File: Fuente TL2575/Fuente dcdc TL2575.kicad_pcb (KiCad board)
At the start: 2 copper layers, 53.3 x 35.6 mm, 20 parts, among them U1 TL2575

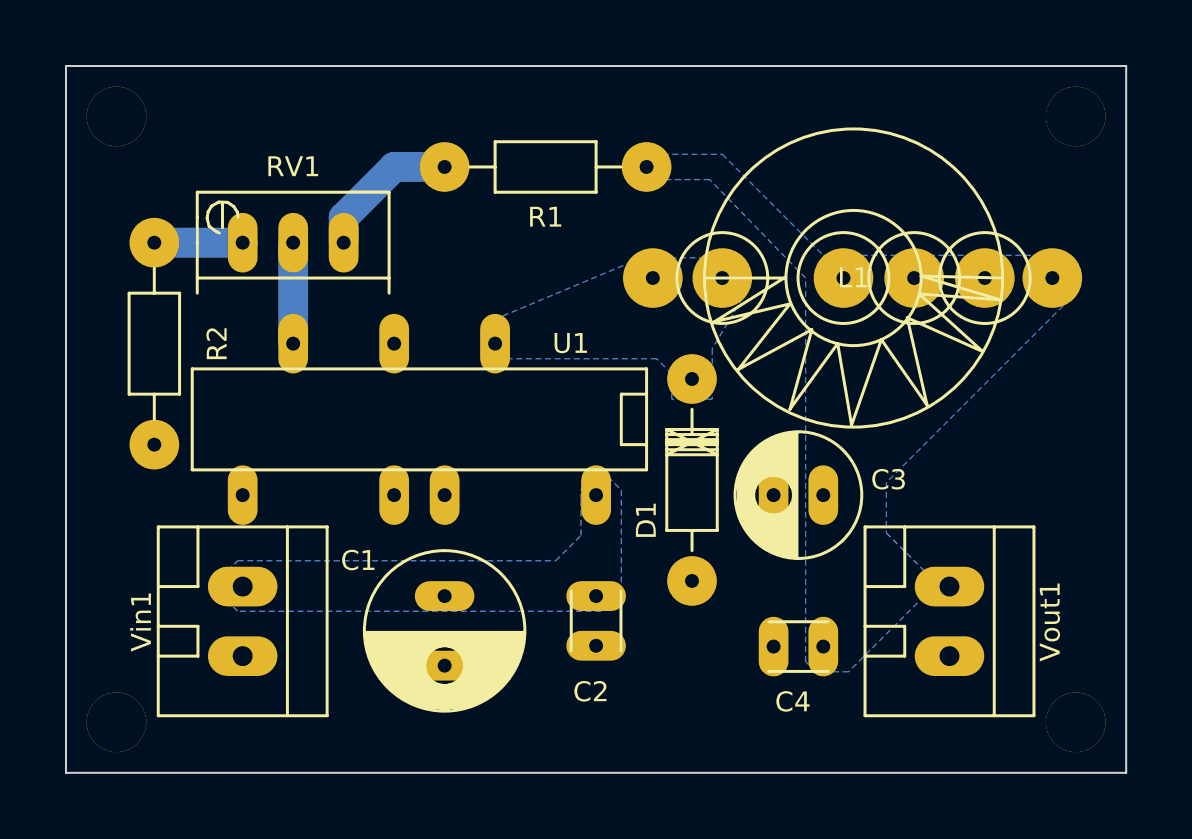
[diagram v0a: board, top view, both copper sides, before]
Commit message: Terminada Fuente TL2575, y controlador
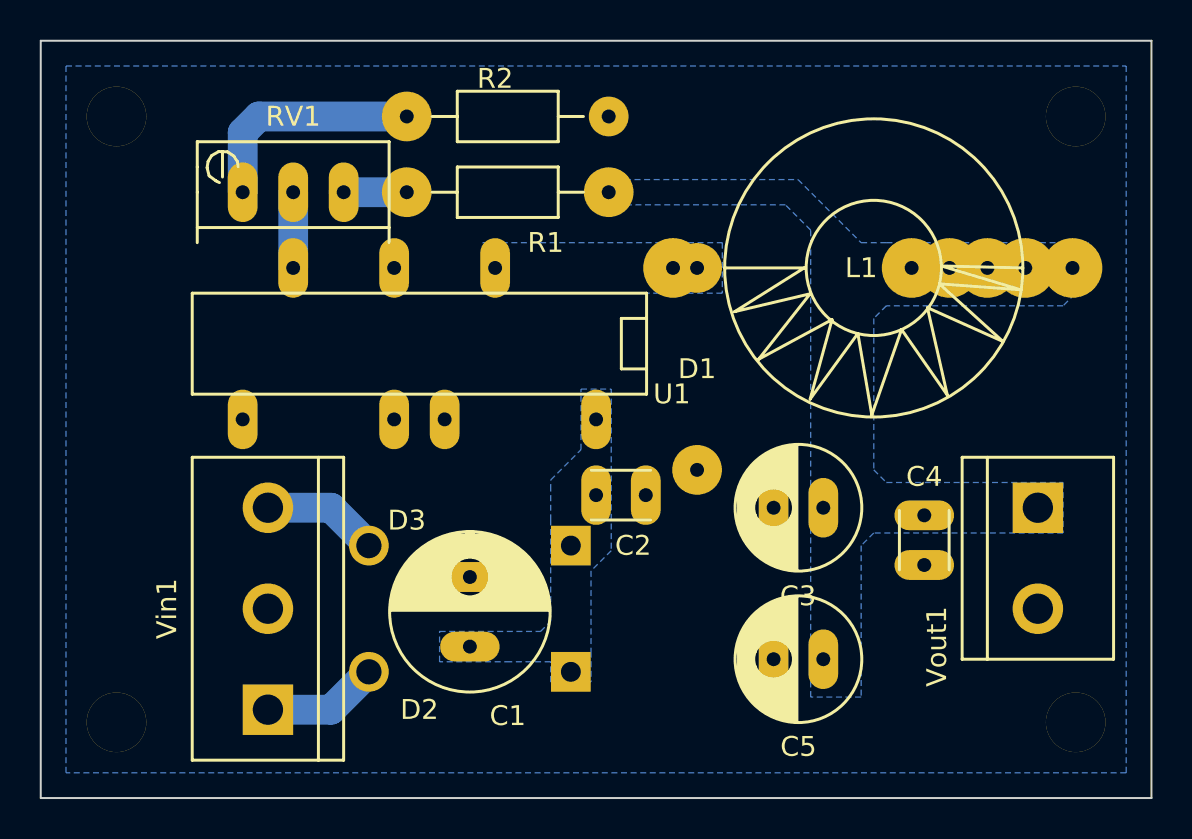
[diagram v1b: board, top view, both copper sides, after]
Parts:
- removed the REF** at (138.2, 48.8)
- removed the REF** at (141.7, 48.8)
- removed the REF** at (145.3, 48.8)
- removed the REF** at (132.1, 48.8)
- added C5: 100uF, Capacitors_ThroughHole:C_Radial_D6.3_L11.2_P2.5, F.Cu at (137.2, 67.9)
- added D2: D, Diodes_ThroughHole:Diode_DO-41_SOD81_Horizontal_RM10, B.Cu at (119.4, 68.6)
- added D3: D, Diodes_ThroughHole:Diode_DO-41_SOD81_Horizontal_RM10, B.Cu at (119.4, 62.2)
- added REF**: 1pin, Connect:1pin, F.Cu at (145.4, 48.3)
- added REF**: 1pin, Connect:1pin, F.Cu at (147.3, 48.3)
- added REF**: 1pin, Connect:1pin, F.Cu at (143.5, 48.3)
- added REF**: 1pin, Connect:1pin, F.Cu at (141.6, 48.3)
- D1: moved to B.Cu
- Vin1: value CONN_01X02 -> CONN_01X03; footprint Sockets_WAGO734:WAGO_734_2pin_Straight_RuggedPads -> Connect:bornier3
- Vout1: footprint Sockets_WAGO734:WAGO_734_2pin_Straight_RuggedPads -> Connect:bornier2
- moved R2 21.1 mm to (121.3, 40.6), turned to 0 degrees
- moved C4 8.33 mm to (142.2, 60.7), turned to 270 degrees
- moved D1 5.59 mm to (130.8, 53.3)
- moved Vout1 5.46 mm to (148.0, 62.9)
- moved C2 5.08 mm to (125.7, 59.7), turned to 0 degrees
- moved U1 3.81 mm to (116.8, 52.1)
- moved C1 2.84 mm to (119.4, 67.3), turned to 90 degrees
- moved RV1 2.54 mm to (108.0, 44.5)
- moved R1 2.29 mm to (121.3, 44.5)
- moved Vin1 1.42 mm to (109.2, 65.4), turned to 90 degrees
- moved L1 1.14 mm to (139.7, 48.3)
- moved C3 0.64 mm to (137.2, 60.3)
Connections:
- Vin1 pad 1: Net-(C1-Pad1) -> Net-(D2-Pad1)
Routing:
- net Net-(R2-Pad1): track 4.45 -> 11.6 mm
- net Net-(D2-Pad1): track 0.00 -> 5.87 mm
- net Net-(D3-Pad1): track 0.00 -> 5.87 mm
- net Net-(R1-Pad2): track 7.40 -> 3.17 mm
- net Net-(RV1-Pad2): track 5.08 -> 3.81 mm
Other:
- board size 53.3 x 35.6 mm -> 55.9 x 38.1 mm

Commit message: Para imprimir, fuente TL2575 y Controlador
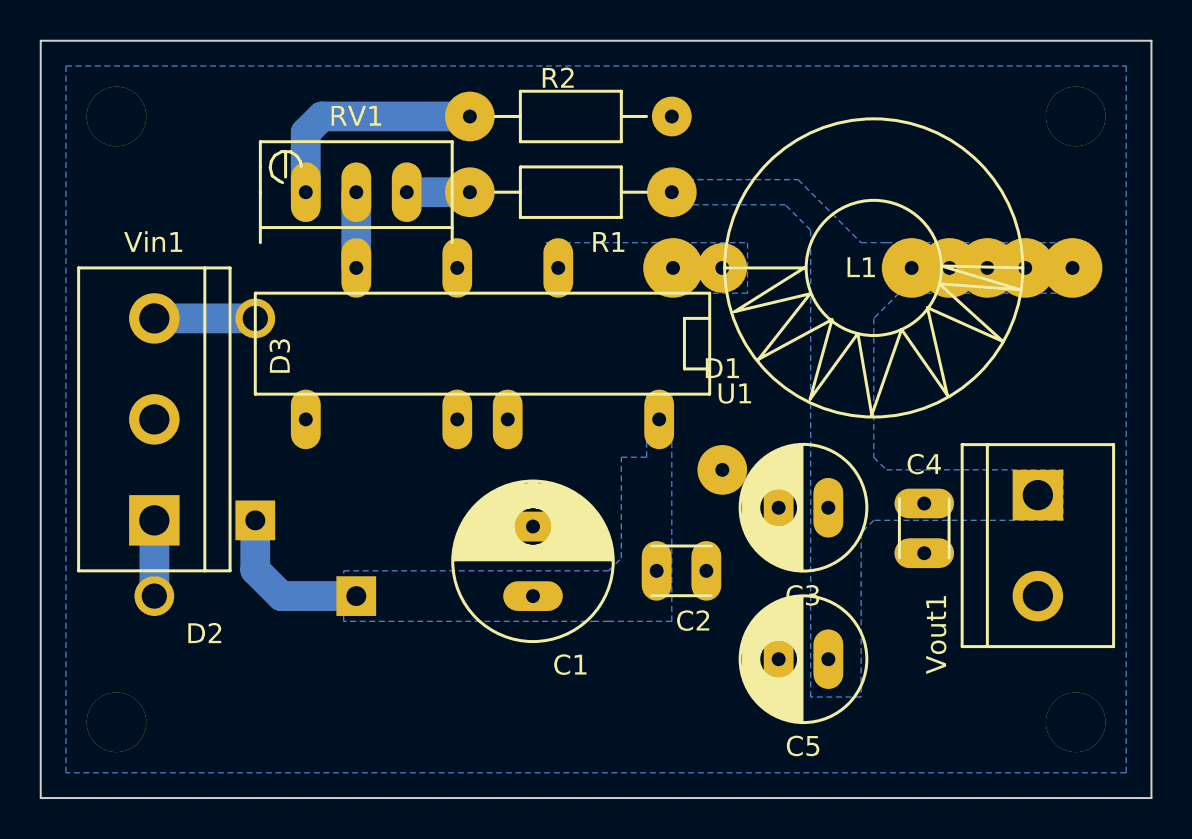
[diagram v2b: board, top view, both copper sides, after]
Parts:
- moved D3 12.5 mm to (108.6, 55.9), turned to 270 degrees
- moved D2 11.4 mm to (108.6, 64.8)
- moved Vin1 11.1 mm to (103.5, 55.9)
- moved C2 4.88 mm to (128.8, 63.5)
- moved C1 4.07 mm to (122.6, 64.8)
- moved R1 3.17 mm to (124.5, 44.5)
- moved R2 3.17 mm to (124.5, 40.6)
- moved RV1 3.17 mm to (111.1, 44.5)
- moved U1 3.17 mm to (120.0, 52.1)
- moved D1 1.27 mm to (132.1, 53.3)
- moved Vout1 0.64 mm to (148.0, 62.2)
- moved C4 0.60 mm to (142.2, 60.1)
- moved C3 0.25 mm to (137.4, 60.3)
- moved C5 0.25 mm to (137.4, 67.9)
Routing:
- net (no net): track 0.00 -> 53.3 mm
- net Net-(C1-Pad1): track 0.00 -> 8.12 mm
- net Net-(D2-Pad1): track 5.87 -> 3.81 mm
- net Net-(D3-Pad1): track 5.87 -> 5.08 mm
